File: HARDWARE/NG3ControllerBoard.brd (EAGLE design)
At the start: 41.6 x 25.1 mm, 10 parts, among them U1 ATMEGA328P-AU, Y1 RESONATORSMD

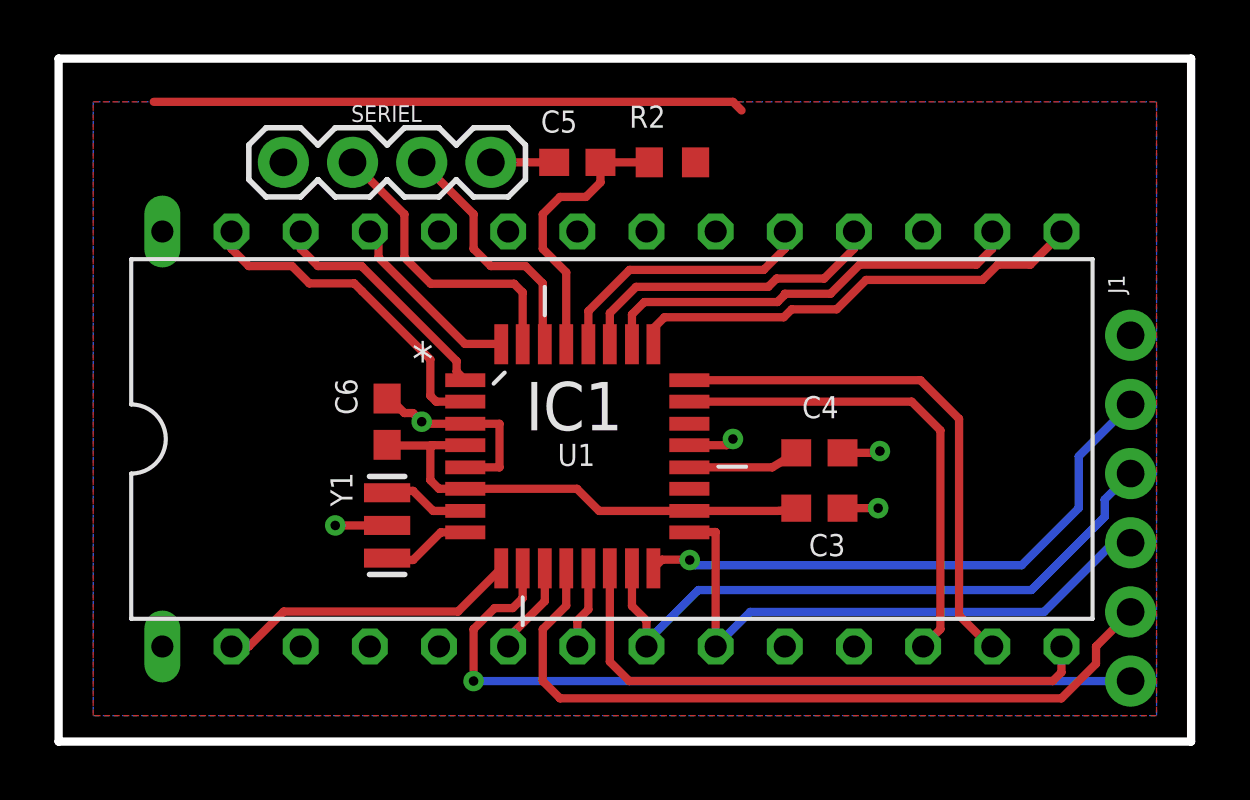
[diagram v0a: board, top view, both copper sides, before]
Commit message: Updated
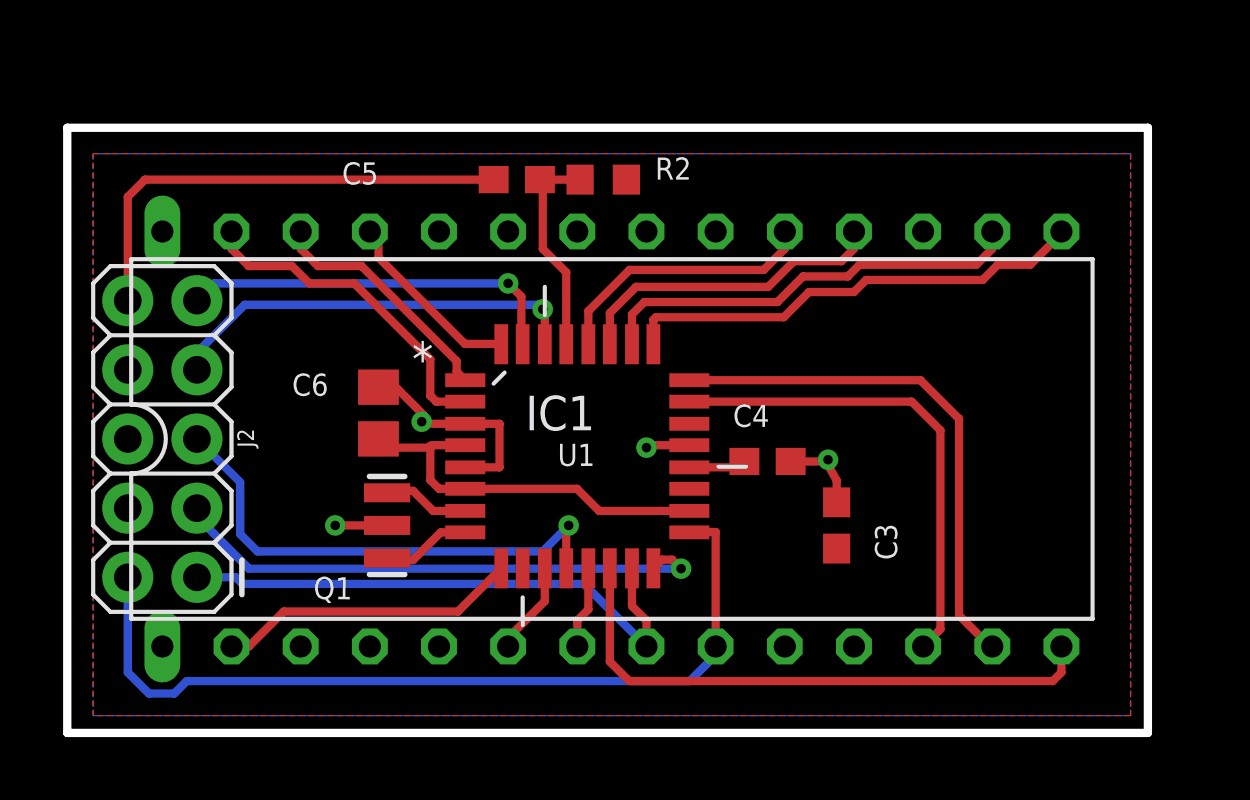
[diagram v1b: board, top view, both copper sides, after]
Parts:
- removed J1: (no value), SparkFun-Connectors:1X06_NO_SILK
- removed SERIEL: (no value), SparkFun-Connectors:1X04
- added J2: (no value), SparkFun-Connectors:2X5
- C3, C4, C5: value (none) -> 100nF
- C6: value (none) -> 1uF; device rcl:C0603 -> rcl:C0805
- Q1: value RESONATORSMD -> 16MHz
- R2: value (none) -> 10K
- moved R2 2.62 mm to (18.7, 19.7)
- moved C5 2.31 mm to (15.6, 19.7)
- moved C4 1.93 mm to (24.8, 9.33)
- moved C3 0.90 mm to (27.3, 6.99), turned to 270 degrees
- moved C6 0.45 mm to (10.5, 11.1)
- renumbered Y1 to Q1
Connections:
- removed net N$1: C5.2, SERIEL.1
- new net DTR: C5.2, J2.10
- net CAN_MSG: no longer J1.6
- net CS_CAN: now also J2.5; no longer J1.5
- net GND: now also J2.6, J2.8; no longer J1.1, SERIEL.4
- net MISO: now also J2.3; no longer J1.2
- net MOSI: now also J2.1; no longer J1.3
- net RXD: now also J2.7; no longer SERIEL.2
- net SCK: now also J2.2; no longer J1.4
- net TXD: now also J2.9; no longer SERIEL.3
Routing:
- net CAN_MSG: track 29.4 -> 0.00 mm, vias 1 -> 0
- net +5V: track 39.9 -> 14.5 mm
- net DTR: track 0.00 -> 17.5 mm
- net CS_CAN: track 28.0 -> 18.5 mm, vias 0 -> 1
- net SCK: track 22.0 -> 31.5 mm
- net RXD: track 9.30 -> 15.6 mm, vias 0 -> 1
- net MOSI: track 24.1 -> 20.8 mm
- net TXD: track 11.1 -> 14.1 mm, vias 0 -> 1
- net RESET: track 10.3 -> 7.92 mm
- net N$1: track 2.32 -> 0.00 mm
- net N$8: track 4.07 -> 2.08 mm
- net GND: track 13.8 -> 15.0 mm, vias 5 -> 4
- net MISO: track 21.3 -> 20.2 mm
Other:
- board size 41.6 x 25.1 mm -> 39.7 x 22.2 mm
